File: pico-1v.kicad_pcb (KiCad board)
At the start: 4 copper layers, 44 parts, among them J2 USB-C-2.0, J3 Header-1, J4 Header-2, J5 SWD, SW1 UK-B0273-SP25Y, SW2 USB Boot, SW4 SW_Slide_DPDT, U1 RP2040, U2 MCP1703Ax-180xxTT, U3 MCP1703Ax-330xxTT, U4 AT25FF161A-SSHN-T, Y1 ECS-3225MV-120-BN-TR3

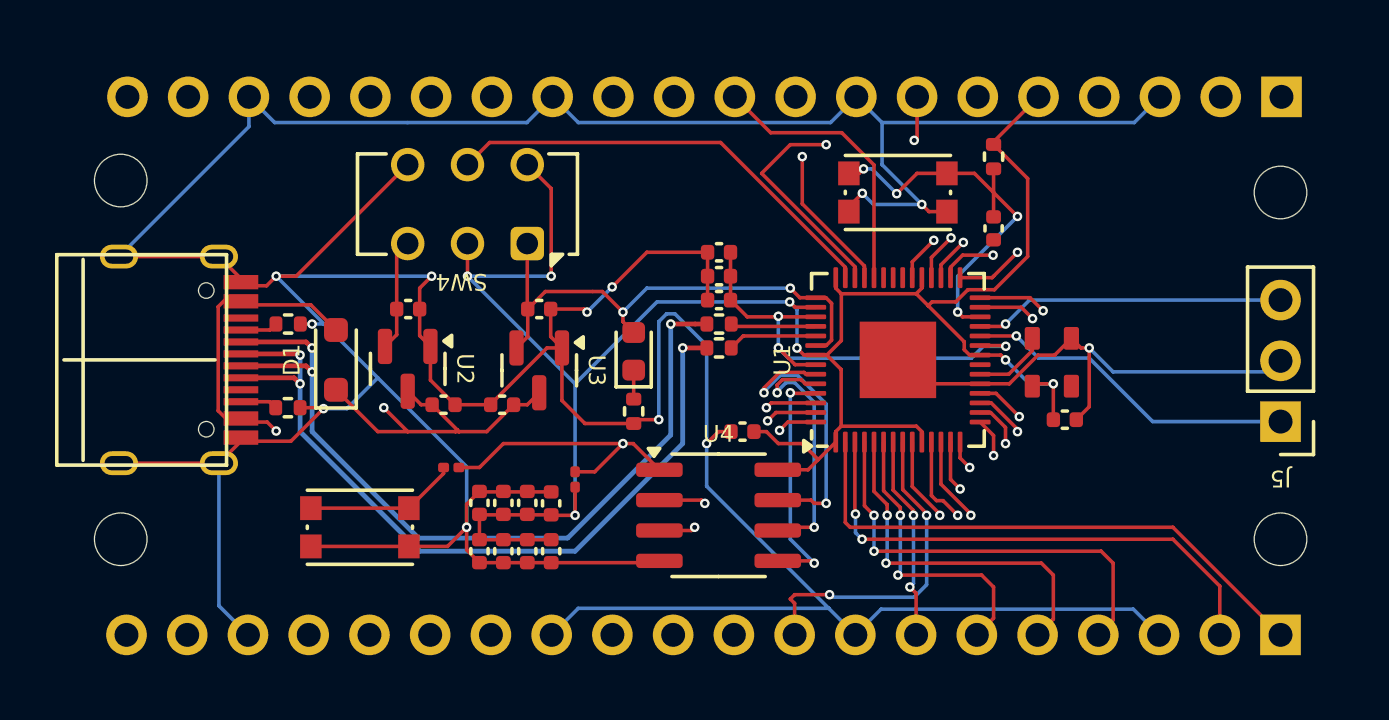
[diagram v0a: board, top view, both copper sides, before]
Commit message: Rev 1 PCB
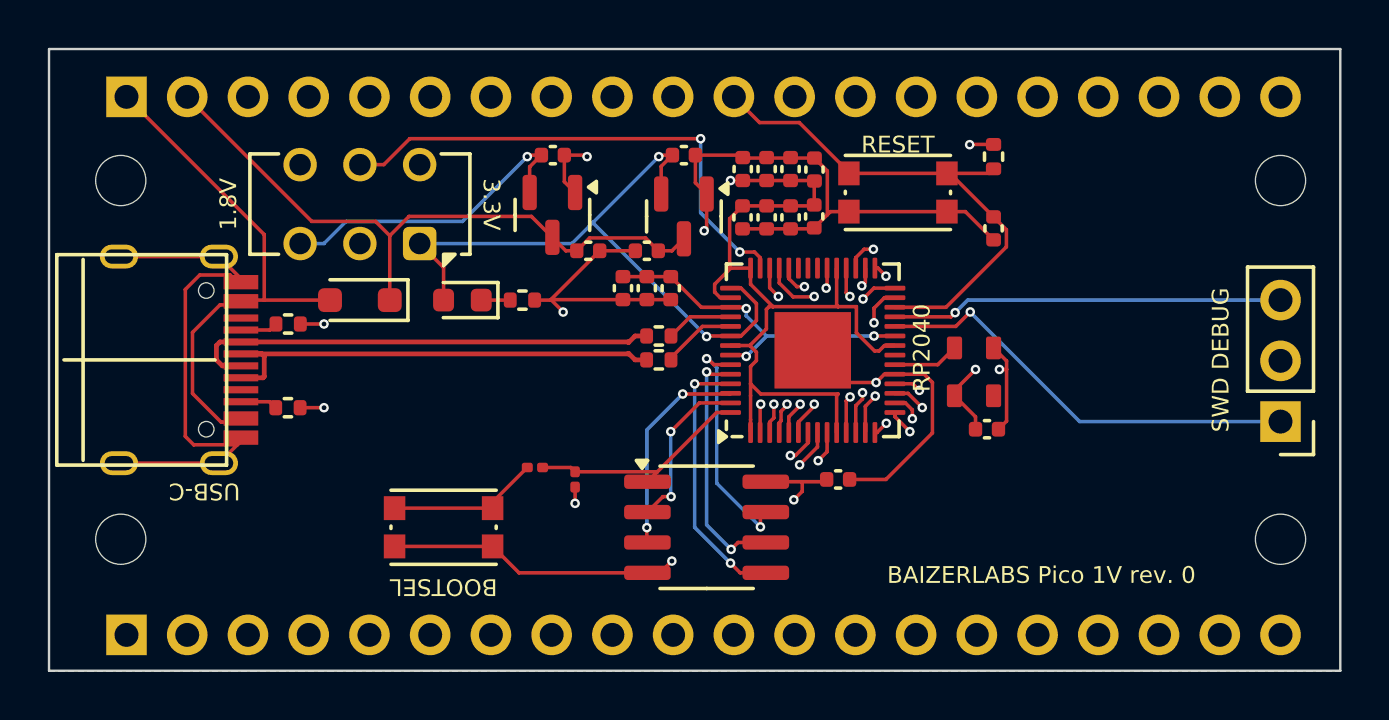
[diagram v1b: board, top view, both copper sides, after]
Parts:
- added G***: LOGO, ExtraFootprints:FireEmoji, B.Cu at (151.0, 96.5)
- H1, H2, H3, H4: footprint MountingHole:MountingHole_2.2mm_M2 -> MountingHole:MountingHole_2.1mm
- moved J4 48.3 mm to (125.2, 85.0), turned to -90 degrees
- moved J3 48.3 mm to (125.2, 107.5), turned to -90 degrees
- moved C8 19.8 mm to (154.0, 90.0)
- moved C10 17.8 mm to (152.0, 88.0)
- moved C11 17.8 mm to (153.0, 88.0)
- moved C9 17.8 mm to (151.0, 88.0)
- moved C12 17.8 mm to (154.0, 88.0)
- moved C6 17.8 mm to (153.0, 90.0)
- moved C7 17.8 mm to (152.0, 90.0)
- moved C5 16.1 mm to (151.0, 90.0)
- moved C13 8.83 mm to (147.0, 91.4)
- moved C15 8.83 mm to (144.6, 91.4)
- moved C16 8.83 mm to (148.6, 87.4)
- moved U2 8.83 mm to (143.1, 89.9)
- moved U3 8.83 mm to (148.6, 90.0)
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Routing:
- net GND: track 235.7 -> 88.7 mm, vias 12 -> 8
- net VDD: track 90.6 -> 44.6 mm, vias 7 -> 5
- net VBUS: track 61.1 -> 22.3 mm, vias 1 -> 0
- net GPIO16: track 57.4 -> 22.6 mm
- net VSYS: track 62.0 -> 27.4 mm, vias 1 -> 0
- net GPIO17: track 51.5 -> 19.9 mm
- net GPIO18: track 42.2 -> 12.6 mm
- net GPIO19: track 37.3 -> 11.7 mm
- net GPIO20: track 33.6 -> 9.49 mm
- net GPIO15: track 44.3 -> 20.5 mm
- net GPIO14: track 41.1 -> 17.8 mm
- net GPIO13: track 34.5 -> 13.5 mm
- net GPIO12: track 30.8 -> 11.8 mm
- net GPIO21: track 29.1 -> 10.7 mm
- net RUN: track 39.8 -> 22.2 mm, vias 4 -> 0
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- added copper zone on B.Cu, net GND
- added copper zone on In2.Cu, net VDD
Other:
- board outline added: 54 x 26 mm
- board text added: "1.8V"
- board text added: "3.3V"
- board text added: "BAIZERLABS Pico 1V rev. 0"
- board text added: "BOOTSEL"
- board text added: "RESET"
- board text added: "RP2040"
- board text added: "SWD DEBUG"
- board text added: "USB-C"
